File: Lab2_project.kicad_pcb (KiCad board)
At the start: 2 copper layers, 129 x 101 mm, 45 parts, among them J1 PROG, J2 POWER IN, SW1 EC11B, SW2 RESET, SW3 BOOT, U1 STM32F407IGTx, U2 AMS1117-3.3, Y1 8 MHz

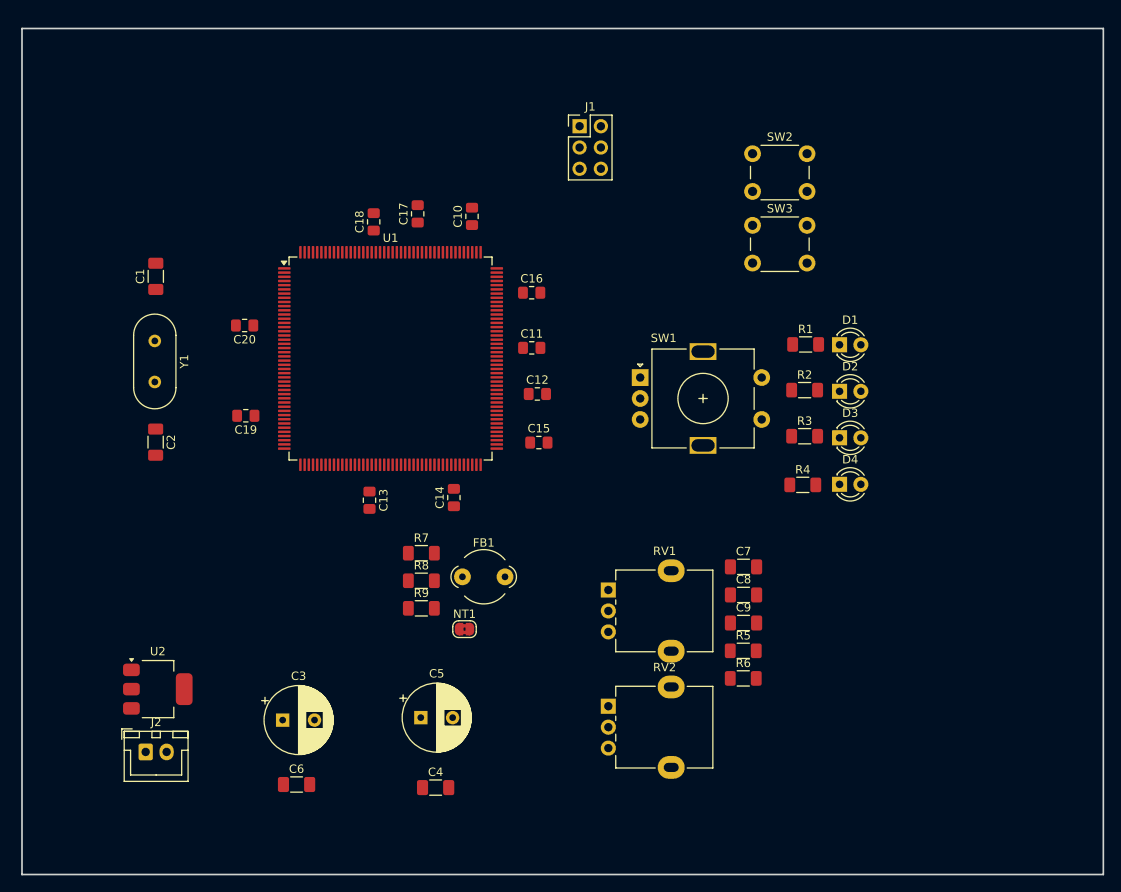
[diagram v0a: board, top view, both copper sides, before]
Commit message: fix: traced PCB
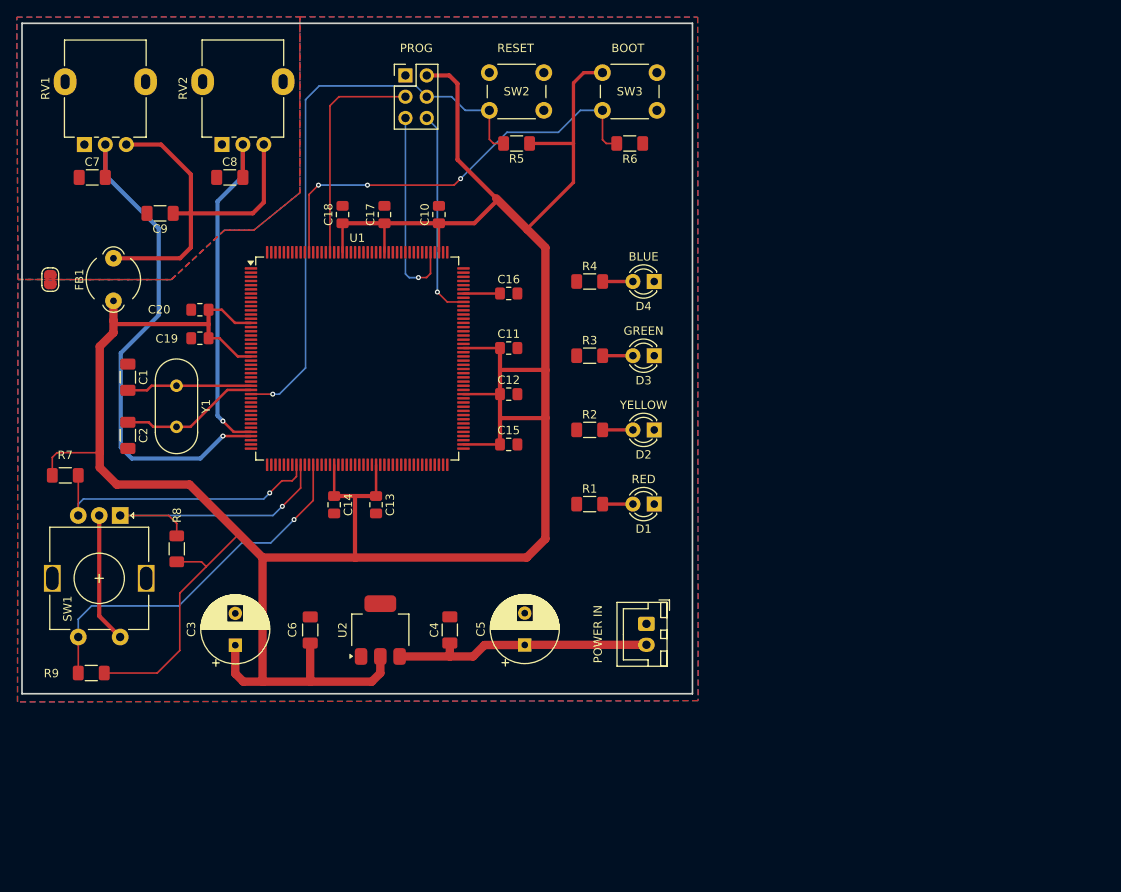
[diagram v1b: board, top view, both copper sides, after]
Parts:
- moved C7 90.5 mm to (102.9, 63.8)
- moved C9 85.1 mm to (111.0, 68.1), turned to 180 degrees
- moved RV1 82.1 mm to (102.0, 59.9), turned to 90 degrees
- moved RV2 81.4 mm to (118.4, 59.9), turned to 90 degrees
- moved C8 79.0 mm to (119.3, 63.8)
- moved R5 66.3 mm to (153.5, 59.8), turned to 180 degrees
- moved R6 65.3 mm to (167.0, 59.8)
- moved NT1 64.7 mm to (97.9, 76.0), turned to 90 degrees
- moved SW1 64.2 mm to (106.2, 104.2), turned to -90 degrees
- moved J2 61.7 mm to (169.0, 117.1), turned to -90 degrees
- moved FB1 53.1 mm to (105.4, 78.5), turned to 90 degrees
- moved R7 43.5 mm to (99.7, 99.4)
- moved R9 40.1 mm to (102.8, 123.0), turned to 180 degrees
- moved R4 35.2 mm to (162.3, 76.2)
- moved D4 32.8 mm to (170.0, 76.2), turned to 180 degrees
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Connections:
- U1 pad 40: RP1 -> RP2
- U1 pad 41: RP2 -> RP1
- U1 pad 52: ENC_CLK -> ENC_DT
- U1 pad 53: ENC_DT -> ENC_CLK
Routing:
- net +3.3V: track 0.00 -> 368.6 mm
- net NRST: track 0.00 -> 69.1 mm, vias 0 -> 1
- net RP1: track 0.00 -> 61.8 mm, vias 0 -> 1
- net BOOT: track 0.00 -> 51.5 mm, vias 0 -> 3
- net +3.3VA: track 0.00 -> 46.0 mm
- net ENC_BTN: track 0.00 -> 44.6 mm, vias 0 -> 1
- net RP2: track 0.00 -> 42.3 mm, vias 0 -> 1
- net ENC_DT: track 0.00 -> 34.9 mm, vias 0 -> 1
- net ENC_CLK: track 0.00 -> 34.3 mm, vias 0 -> 1
- net +5V: track 0.00 -> 31.6 mm
- net SWO: track 0.00 -> 26.9 mm
- net SWDIO: track 0.00 -> 24.9 mm, vias 0 -> 1
- net SWCLK: track 0.00 -> 24.6 mm, vias 0 -> 1
- net OSC_OUT: track 0.00 -> 16.7 mm
- net GND: track 0.00 -> 15.5 mm
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- added copper zone on B.Cu, net GND
- added copper zone on F.Cu, net GND
- added copper zone on B.Cu, net GNDA
- added copper zone on F.Cu, net GNDA
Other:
- board size 129 x 101 mm -> 80 x 80 mm
